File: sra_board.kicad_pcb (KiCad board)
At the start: 2 copper layers, 90 x 78.1 mm, 164 parts, among them J1 Conn_01x14_Pin, J10 Conn_01x03_Pin, J11 Conn_01x03_Pin, J12 Conn_01x03_Pin, J13 MPU0650, J14 LSA, J15 OLED, J16 Conn_01x03_Pin, J17 Conn_01x03_Pin, J18 Conn_01x03_Pin, J3 Conn_01x08_Pin, J4 Conn_01x14_Pin, J5 USB_C_Receptacle_USB2.0_16P, J6 B2B-XH-A_LF__SN_, J7 B2B-XH-A_LF__SN_, J8 B2B-XH-A_LF__SN_, J9 Conn_01x03_Pin, Q1 SS8050, Q2 SS8050, Q3 AO3400A, Q4 AO3401A, Q5 AO3401A, Q6 AO3401A, Q7 AO3401A, SW1 SW_0, SW2 SW_EN, SW3 Switch, SW4 Switch, SW5 SW_Wuerth_450301014042, SW6 SW_Wuerth_450301014042, U1 MAX7219CWG_T, U2 CH340C, U3 TB6612FNG H-bridge Motor Driv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, U5 CN3303, U6 TPS562202, U7 ME6211C33M5, U8 ESP32-WROOM-32E

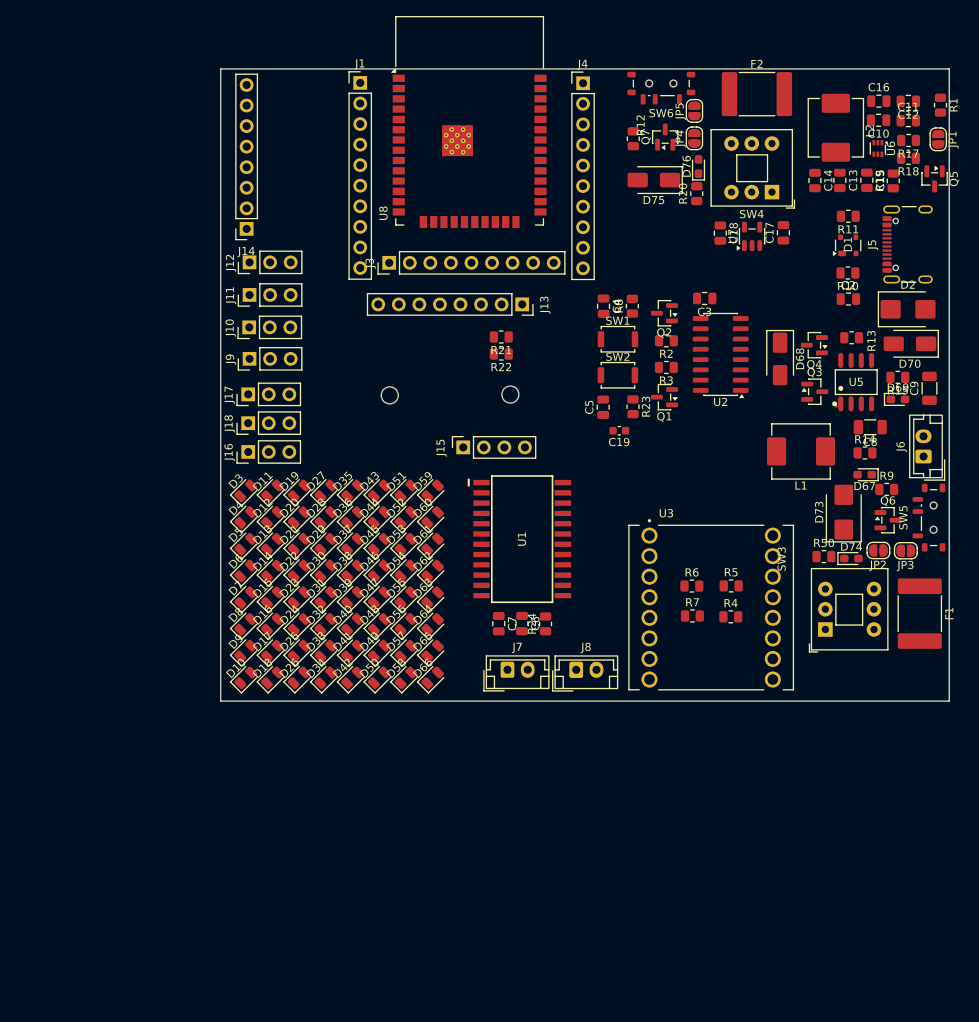
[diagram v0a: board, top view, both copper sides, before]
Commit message: Finishing the routing
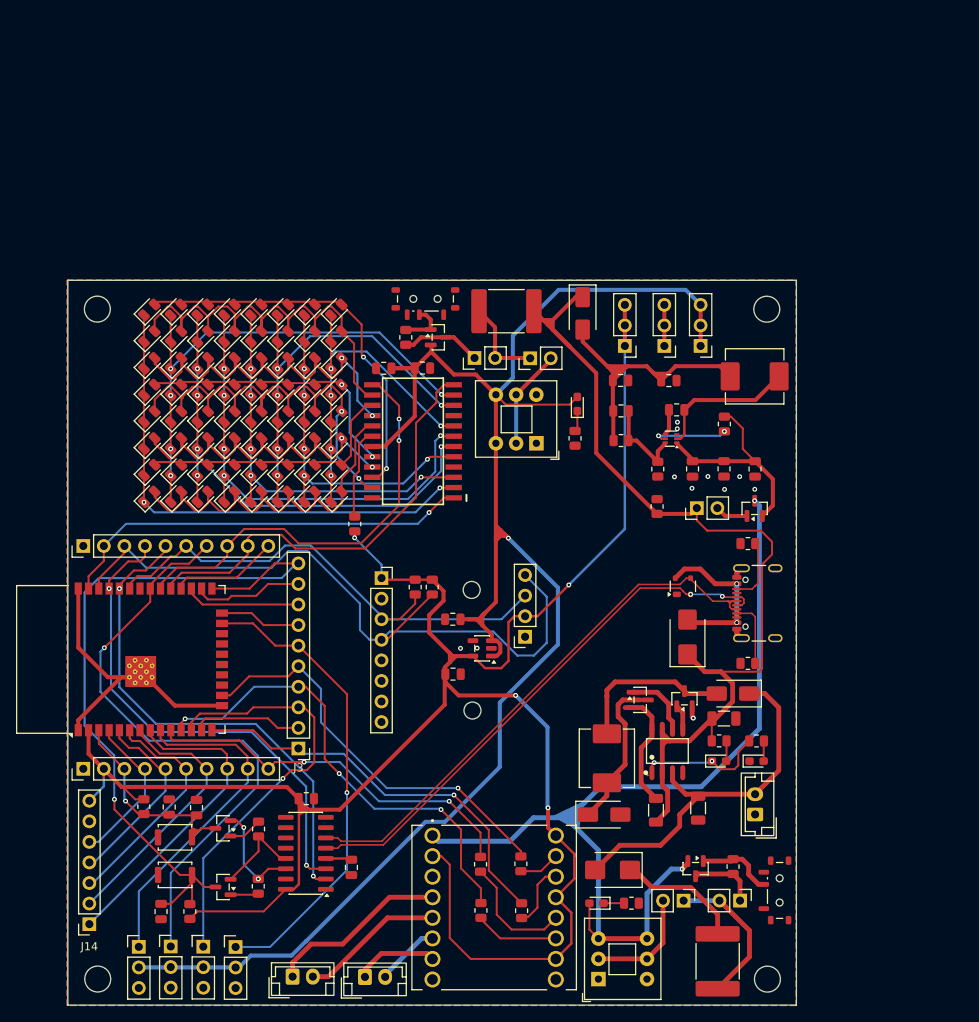
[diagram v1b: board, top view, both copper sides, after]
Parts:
- added ?: , , F.Cu at (200.8, 136.2)
- added ?: , , F.Cu at (118.0, 136.2)
- added H1: MountingHole, MountingHole:MountingHole_3.2mm_M3, F.Cu at (200.7, 53.5)
- added H4: MountingHole, MountingHole:MountingHole_3.2mm_M3, F.Cu at (118.0, 53.5)
- C19: footprint Capacitor_SMD:C_0603_1608Metric -> Capacitor_SMD:C_0805_2012Metric
- J14: footprint Connector_PinSocket_2.54mm:PinSocket_1x08_P2.54mm_Vertical -> Connector_PinSocket_2.54mm:PinSocket_1x07_P2.54mm_Vertical
- J3: footprint Connector_PinHeader_2.54mm:PinHeader_1x09_P2.54mm_Vertical -> Connector_PinHeader_2.54mm:PinHeader_1x10_P2.54mm_Vertical
- JP1, JP2, JP3, JP4, JP5: footprint Jumper:SolderJumper-2_P1.3mm_Open_RoundedPad1.0x1.5mm -> Connector_PinHeader_2.54mm:PinHeader_1x02_P2.54mm_Vertical
- R13: footprint Resistor_SMD:R_0805_2012Metric -> Resistor_SMD:R_1206_3216Metric
- moved C2 93.3 mm to (149.4, 122.4), turned to -90 degrees
- moved R8 92.6 mm to (129.4, 127.9), turned to -90 degrees
- moved C4 92.6 mm to (125.8, 127.9), turned to 90 degrees
- moved J1 91.4 mm to (116.2, 110.3), turned to 90 degrees
- moved Q2 89.4 mm to (133.5, 124.9)
- moved J14 88.1 mm to (117.0, 129.5)
- moved SW1 85.9 mm to (127.6, 123.4)
- moved J12 85.1 mm to (127.0, 132.2), turned to 0 degrees
- moved J4 84.1 mm to (116.2, 82.7), turned to 90 degrees
- moved J11 81.7 mm to (123.1, 132.3), turned to 0 degrees
- moved R3 81.5 mm to (137.8, 124.8), turned to -90 degrees
- moved U2 80.2 mm to (143.7, 120.7)
- moved SW2 79.1 mm to (127.6, 118.7)
- moved C3 79.0 mm to (143.8, 114.0), turned to 0 degrees
- moved R2 78.6 mm to (137.9, 117.7), turned to 90 degrees
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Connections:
- net /7V4_Switch renamed /12V_Switch
- net /7v4 renamed /12V
- J3 pad 6: /2 -> /15
- J3 pad 7: /16 -> /2
- J3 pad 8: /4 -> /16
- J3 pad 9: /0 -> /4
- J4 pad 2: /Din -> /23
- J4 pad 8: /CLK -> /18
- J4 pad 9: /CS -> /5
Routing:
- net /3V3: track 0.00 -> 256.3 mm, vias 0 -> 4
- net /5V_P: track 0.00 -> 218.7 mm, vias 0 -> 1
- net /5V_P_USB: track 0.00 -> 124.1 mm
- net /12V: track 0.00 -> 114.4 mm, vias 0 -> 2
- net /0: track 0.00 -> 93.6 mm, vias 0 -> 1
- net /22: track 0.00 -> 86.9 mm
- net /19: track 0.00 -> 75.5 mm, vias 0 -> 1
- net /D-: track 0.00 -> 68.4 mm
- net /D+: track 0.00 -> 67.0 mm, vias 0 -> 2
- net /21: track 0.00 -> 63.3 mm
- net /C1: track 0.00 -> 63.1 mm, vias 0 -> 2
- net /C2: track 0.00 -> 63.1 mm, vias 0 -> 5
- net /C3: track 0.00 -> 63.0 mm, vias 0 -> 5
- net /TXD: track 0.00 -> 61.9 mm, vias 0 -> 2
- net /R2: track 0.00 -> 61.8 mm
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- added copper zone on B.Cu, net GND
- added copper zone on F.Cu, net GND
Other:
- board size 90 x 78.1 mm -> 90 x 89.5 mm
